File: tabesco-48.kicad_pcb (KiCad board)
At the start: 2 copper layers, 192.5 x 118.4 mm, 98 parts, among them SW1 SW_Push, U1 ProMicro

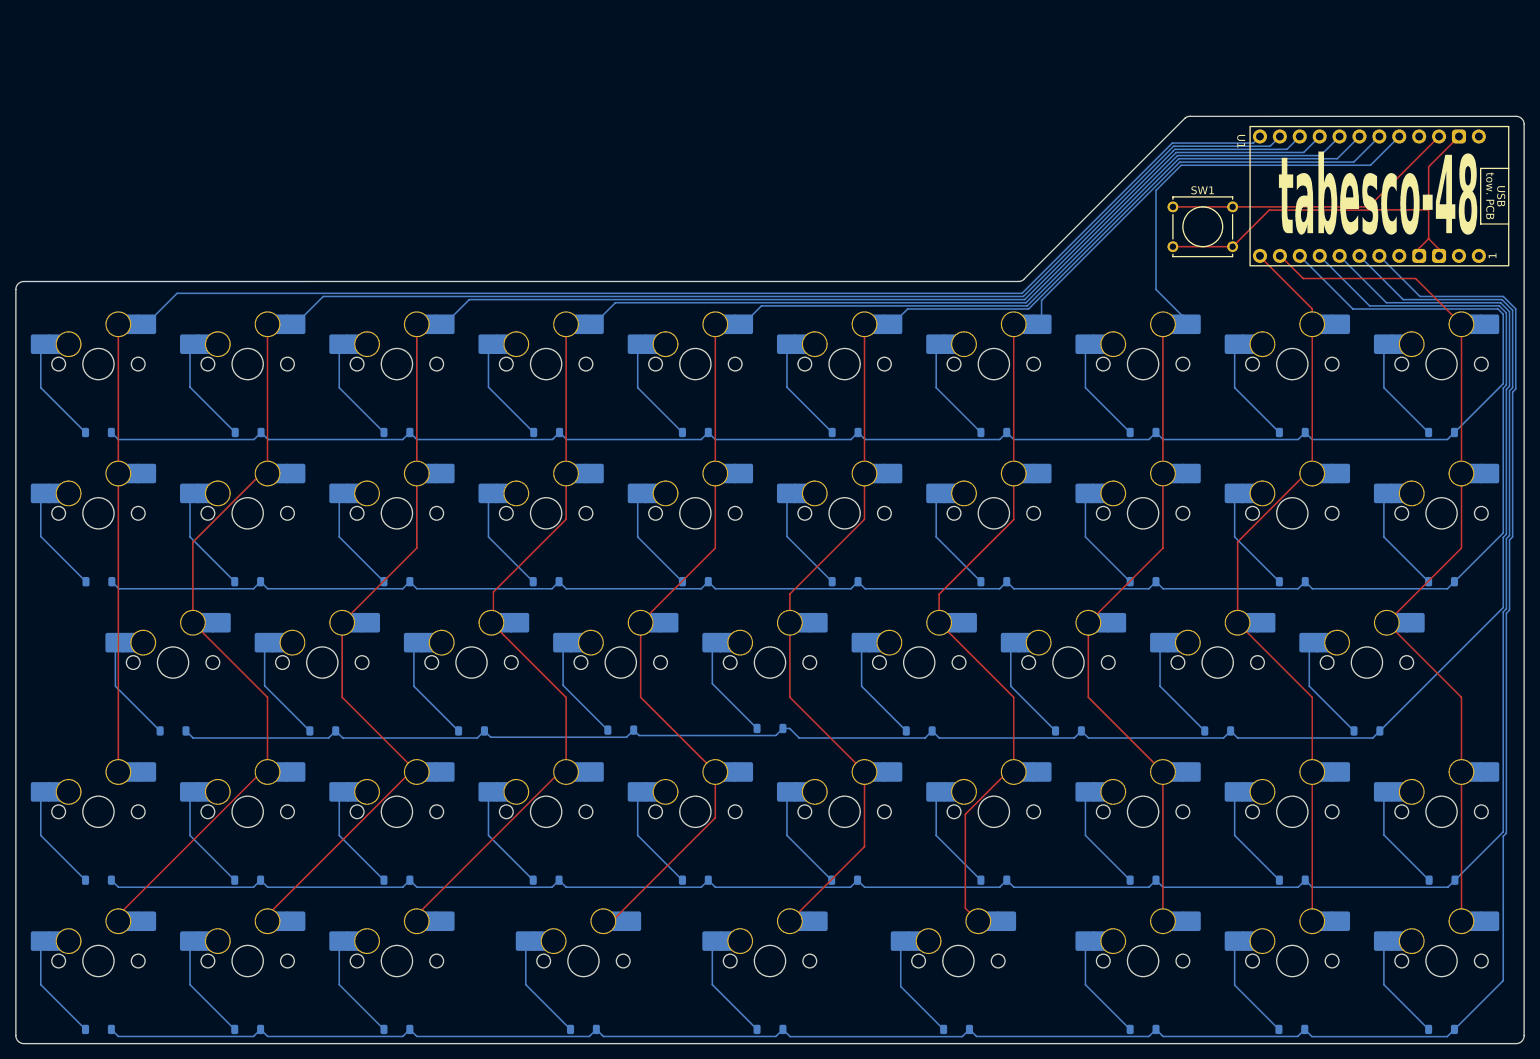
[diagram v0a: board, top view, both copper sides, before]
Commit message: created 6 key tapdance pad 2007 rot brains stupid
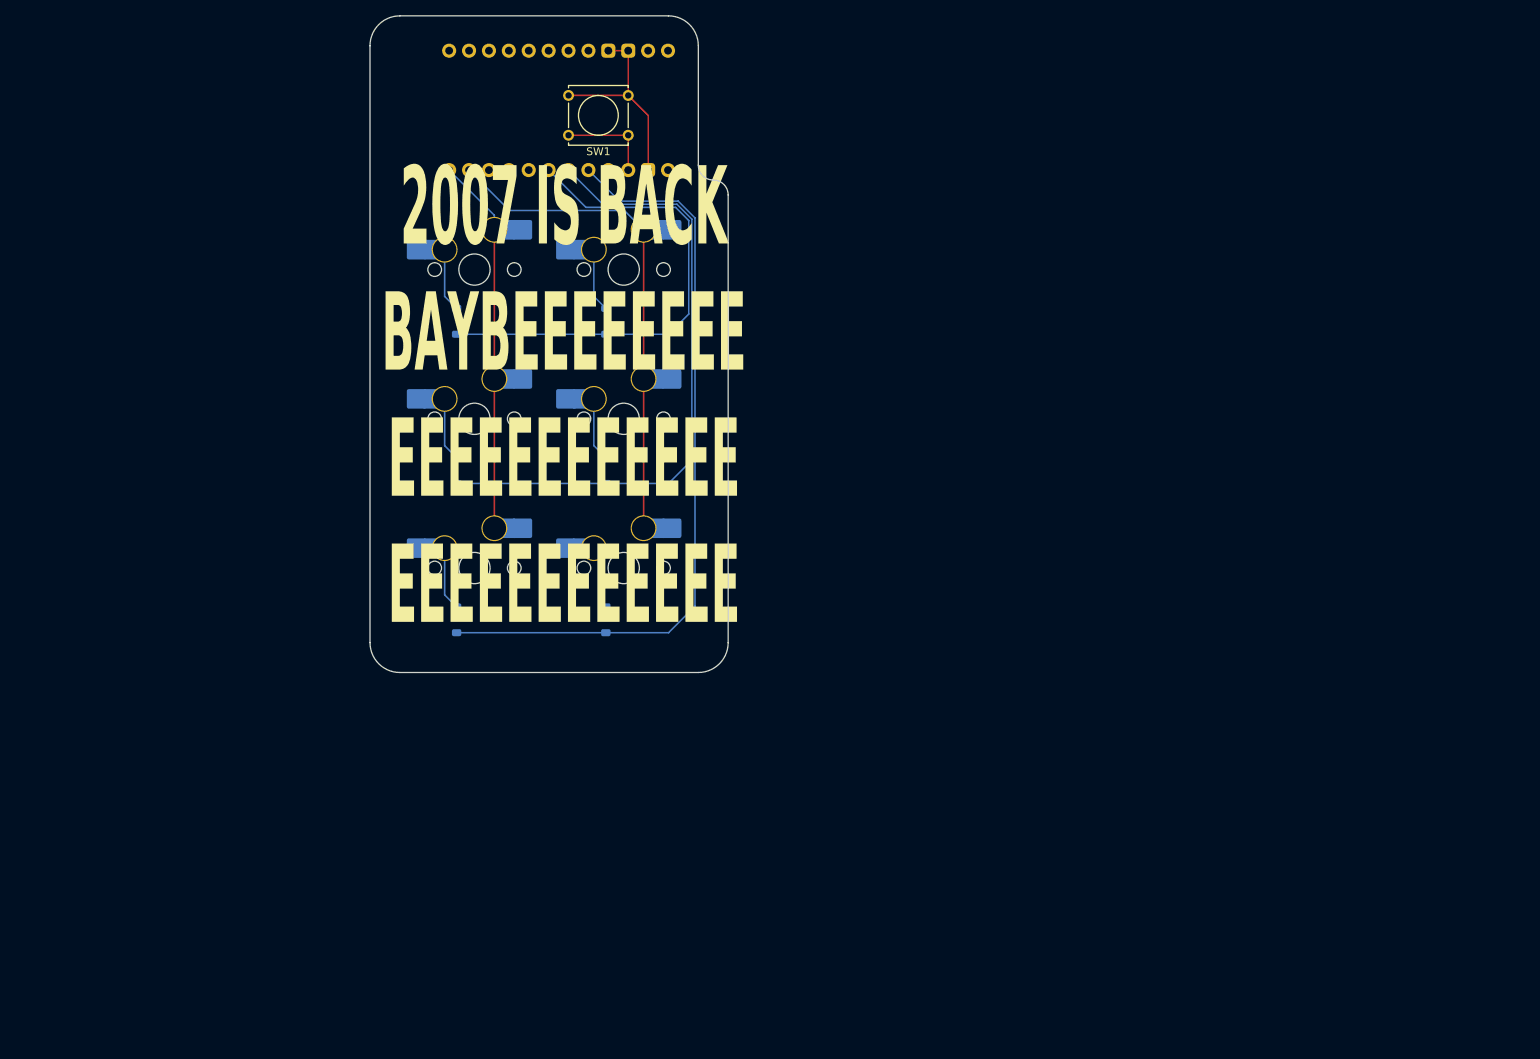
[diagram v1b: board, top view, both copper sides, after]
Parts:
- removed D10, D11, D12, D13, D14, D15, D16, D17, D18, D19, D20, D21, D22, D23, D24, D25, D26, D27, D28, D29, D30, D31, D32, D33, D34, D35, D36, D37, D38, D39, D40, D41, D42, D43, D44, D45, D46, D47, D48, D7, D8, D9: D_Small, Diode_SMD:D_SOD-123
- removed MX10, MX11, MX12, MX13, MX14, MX15, MX16, MX17, MX18, MX19, MX20, MX21, MX22, MX23, MX24, MX25, MX26, MX27, MX28, MX29, MX30, MX31, MX32, MX33, MX34, MX35, MX36, MX37, MX38, MX39, MX40, MX41, MX42, MX43, MX44, MX45, MX46, MX47, MX48, MX7, MX8, MX9: MX_SW_HS, marbastlib-mx:SW_MX_HS_CPG151101S11_1u
- U1: moved to B.Cu
- moved D1 126.5 mm to (115.2, 52.5), turned to 90 degrees
- moved MX1 124.0 mm to (117.5, 45.8)
- moved U1 104.1 mm to (128.2, 25.5), turned to 90 degrees
- moved D2 88.8 mm to (134.2, 52.5), turned to 90 degrees
- moved D3 87.8 mm to (115.2, 71.5), turned to 90 degrees
- moved MX2 86.2 mm to (136.5, 45.8)
- moved MX3 85.6 mm to (117.5, 64.9)
- moved SW1 70.1 mm to (137.1, 28.7), turned to 180 degrees
- moved D5 55.1 mm to (115.2, 90.6), turned to 90 degrees
- moved MX5 53.9 mm to (117.5, 83.9)
- moved D4 49.8 mm to (134.2, 71.5), turned to 90 degrees
- moved MX4 47.8 mm to (136.5, 64.9)
- moved MX6 27.6 mm to (136.5, 83.9)
- moved D6 26.5 mm to (134.2, 90.6), turned to 90 degrees
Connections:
- D3 pad 1: /row0 -> /row1
- D4 pad 1: /row0 -> /row1
- D5 pad 1: /row0 -> /row2
- D6 pad 1: /row0 -> /row2
- MX3 pad 2: /col2 -> /col0
- MX4 pad 2: /col3 -> /col1
- MX5 pad 2: /col4 -> /col0
- MX6 pad 2: /col5 -> /col1
- U1 pad 10: /row0 -> unconnected-(U1-E6-Pad10)
- U1 pad 11: /col0 -> unconnected-(U1-B4-Pad11)
- U1 pad 12: /col1 -> unconnected-(U1-B5-Pad12)
- U1 pad 17: /col2 -> /row2
- U1 pad 18: /col3 -> /row1
- U1 pad 19: /col4 -> /row0
- U1 pad 20: /col5 -> unconnected-(U1-F7-Pad20)
- U1 pad 21: /col6 -> unconnected-(U1-B1-Pad21)
- U1 pad 22: /col7 -> unconnected-(U1-B3-Pad22)
- U1 pad 23: /col8 -> /col1
- U1 pad 24: /col9 -> /col0
- U1 pad 6: /row4 -> unconnected-(U1-D0-Pad6)
- U1 pad 7: /row3 -> unconnected-(U1-D4-Pad7)
- U1 pad 8: /row2 -> unconnected-(U1-C6-Pad8)
- U1 pad 9: /row1 -> unconnected-(U1-D7-Pad9)
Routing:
- net /row4: track 292.9 -> 0.00 mm
- net /row3: track 276.5 -> 0.00 mm
- net /col8: track 228.5 -> 0.00 mm
- net /col7: track 211.5 -> 0.00 mm
- net /col9: track 209.3 -> 0.00 mm
- net /col6: track 195.2 -> 0.00 mm
- net /col5: track 176.7 -> 0.00 mm
- net /row0: track 224.9 -> 63.2 mm
- net /row1: track 242.0 -> 80.4 mm
- net /col4: track 157.6 -> 0.00 mm
- net /row2: track 243.4 -> 97.5 mm
- net /col3: track 142.6 -> 0.00 mm
- net /col2: track 136.9 -> 0.00 mm
- net /col0: track 111.3 -> 48.1 mm
- net /col1: track 96.1 -> 63.5 mm
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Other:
- board size 192.5 x 118.4 mm -> 45.7 x 83.8 mm
- board text added: "2007 IS BACK BAYBEEEEEEEE EEEEEEEEEEEE EEEEEEEEEEEE"
- board text added: "this keypad is for MYSPACE ONLY!!! >.< rawRRRR R"
- board text removed: "tabesco-48"
